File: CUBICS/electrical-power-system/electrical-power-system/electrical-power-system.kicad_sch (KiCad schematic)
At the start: 24 parts, among them J101 Conn_01x02, J102 Conn_01x02, J103 Conn_01x02, J104 Conn_01x02, J105 Conn_01x05, J106 Conn_01x05, J107 Conn_01x05, J108 Conn_01x05, J109 Conn_01x05, J110 Conn_01x05

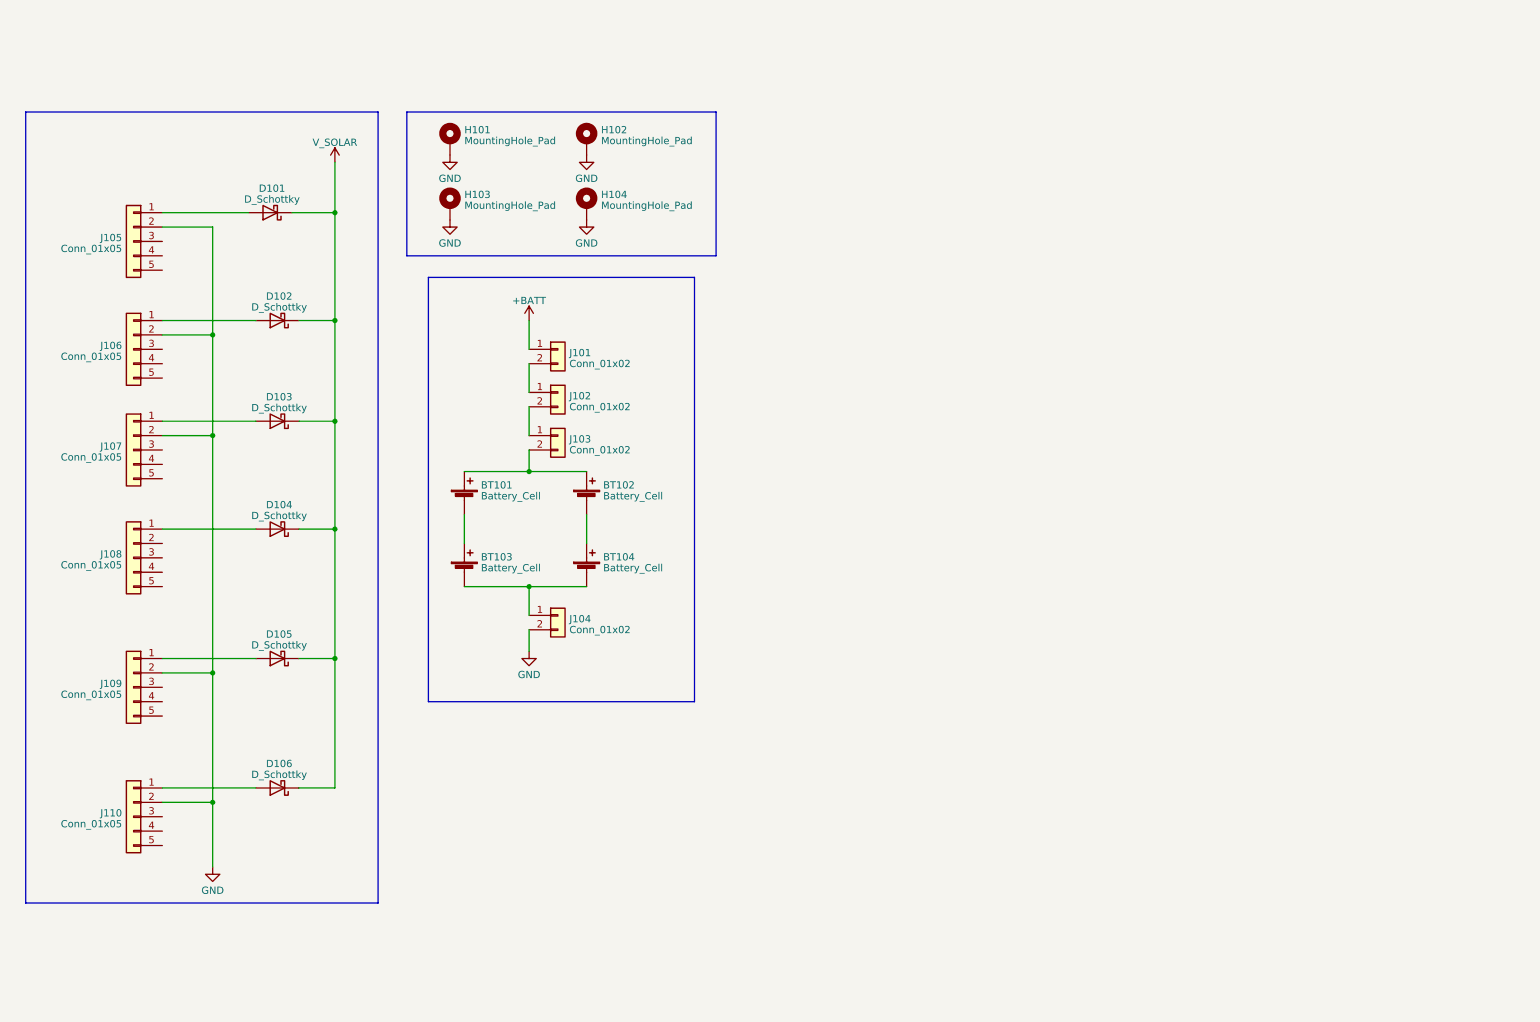
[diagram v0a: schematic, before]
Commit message: schematic v1.0
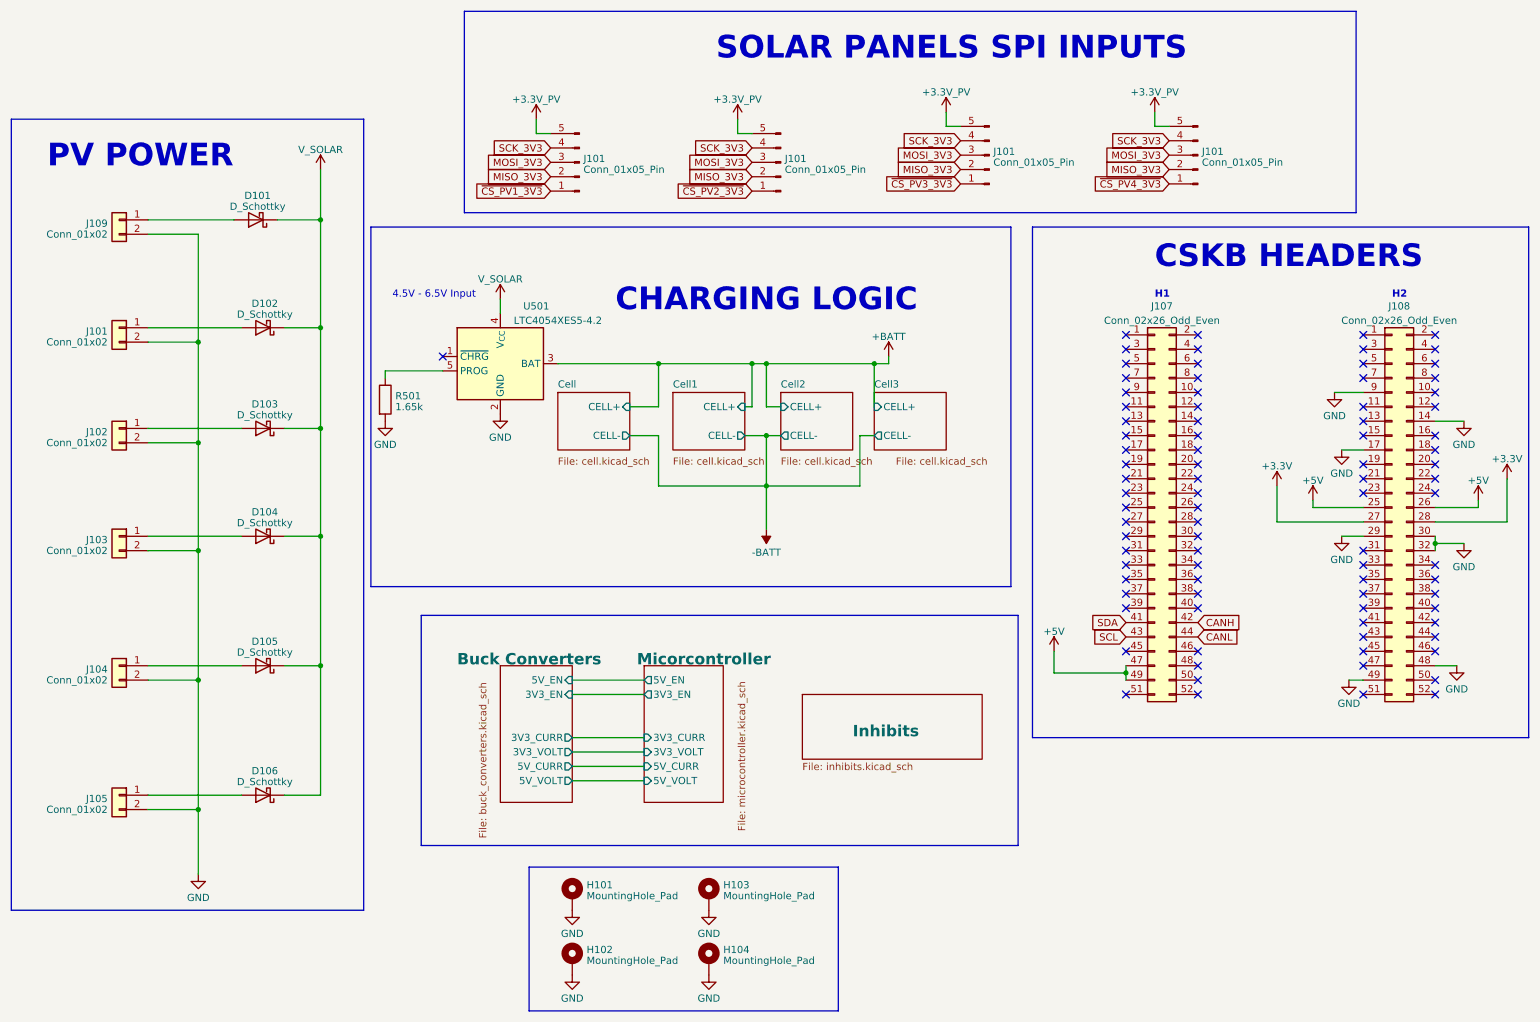
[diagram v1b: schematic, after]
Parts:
- removed BT101, BT102, BT103, BT104: Battery_Cell, symbol Device:Battery_Cell
- removed J105, J106, J107, J108, J109, J110: Conn_01x05, symbol Connector_Generic:Conn_01x05
- added J101 (x4): Conn_01x05_Pin, Connector_Hirose:Hirose_DF13-05P-1.25DSA_1x05_P1.25mm_Vertical, symbol Connector:Conn_01x05_Pin
- added J105, J109: Conn_01x02, symbol Connector_Generic:Conn_01x02
- added J107, J108: Conn_02x26_Odd_Even, Connector_PinSocket_2.54mm:PinSocket_2x26_P2.54mm_Vertical, symbol Connector_Generic:Conn_02x26_Odd_Even
- added R501: 1.65k, symbol Device:R
- added U501: LTC4054XES5-4.2, Package_TO_SOT_SMD:TSOT-23-5, symbol Battery_Management:LTC4054XES5-4.2
- renumbered H103 to H102, H102 to H103
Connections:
- net +1V2: now also U501.4 (V_{CC})
- net +BATT: now also U501.3 (BAT); no longer J101.1 (Pin_1)
- net GND: now also J101.2 (Pin_2), J102.2 (Pin_2), J103.2 (Pin_2), J105.2 (Pin_2), J108.14 (Pin_14), J108.17 (Pin_17), J108.29 (Pin_29), J108.30 (Pin_30), J108.32 (Pin_32), J108.48 (Pin_48), J108.49 (Pin_49), J108.9 (Pin_9), J109.2 (Pin_2), R501.2, U501.2 (GND)
- net at D106.2 (A): now also J105.1 (Pin_1)
- net at D101.2 (A): now also J109.1 (Pin_1)
- net at D104.2 (A): now also J103.1 (Pin_1)
- net at D102.2 (A): now also J101.1 (Pin_1)
- net at J104.1 (Pin_1): now also D105.2 (A)
- net at J102.1 (Pin_1): now also D103.2 (A); no longer J101.2 (Pin_2)
- new net: R501.1, U501.5 (PROG)
- new net +3.3V: J101.5 (Pin_5), J101.5 (Pin_5), J101.5 (Pin_5), J101.5 (Pin_5), J108.27 (Pin_27), J108.28 (Pin_28)
- new net +5V: J107.47 (Pin_47), J107.49 (Pin_49), J108.25 (Pin_25), J108.26 (Pin_26)
- new net CANH: J107.42 (Pin_42)
- new net CANL: J107.44 (Pin_44)
- new net MISO_3V3: J101.2 (Pin_2), J101.2 (Pin_2), J101.2 (Pin_2), J101.2 (Pin_2)
- new net MOSI_3V3: J101.3 (Pin_3), J101.3 (Pin_3), J101.3 (Pin_3), J101.3 (Pin_3)
- new net SCK_3V3: J101.4 (Pin_4), J101.4 (Pin_4), J101.4 (Pin_4), J101.4 (Pin_4)
- new net SCL: J107.43 (Pin_43)
- new net SDA: J107.41 (Pin_41)
- new net ~{CS_PV1_3V3}: J101.1 (Pin_1)
- new net ~{CS_PV2_3V3}: J101.1 (Pin_1)
- new net ~{CS_PV3_3V3}: J101.1 (Pin_1)
- new net ~{CS_PV4_3V3}: J101.1 (Pin_1)
- no-connect marks 0 -> 87
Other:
- added sheet Buck Converters (buck_converters.kicad_sch)
- added sheet Cell (cell.kicad_sch)
- added sheet Cell1 (cell.kicad_sch)
- added sheet Cell2 (cell.kicad_sch)
- added sheet Cell3 (cell.kicad_sch)
- added sheet Inhibits (inhibits.kicad_sch)
- added sheet Micorcontroller (microcontroller.kicad_sch)
- note added: "4.5V - 6.5V Input"
- note added: "CHARGING LOGIC"
- note added: "CSKB HEADERS"
- note added: "H1"
- note added: "H2"
- note added: "PV POWER"
- note added: "SOLAR PANELS SPI INPUTS"
- moved on the sheet: D101, D102, D103, D104, D105, D106, H101, H102, H103, H104
